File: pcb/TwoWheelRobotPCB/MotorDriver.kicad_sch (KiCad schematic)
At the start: 23 parts, among them J1 L298n_sense_connector, J2 ACS712_connector, J3 Motor1, J4 Motor2, U2 L298HN, U3 PCF8574, U4 TXB0108DQSR

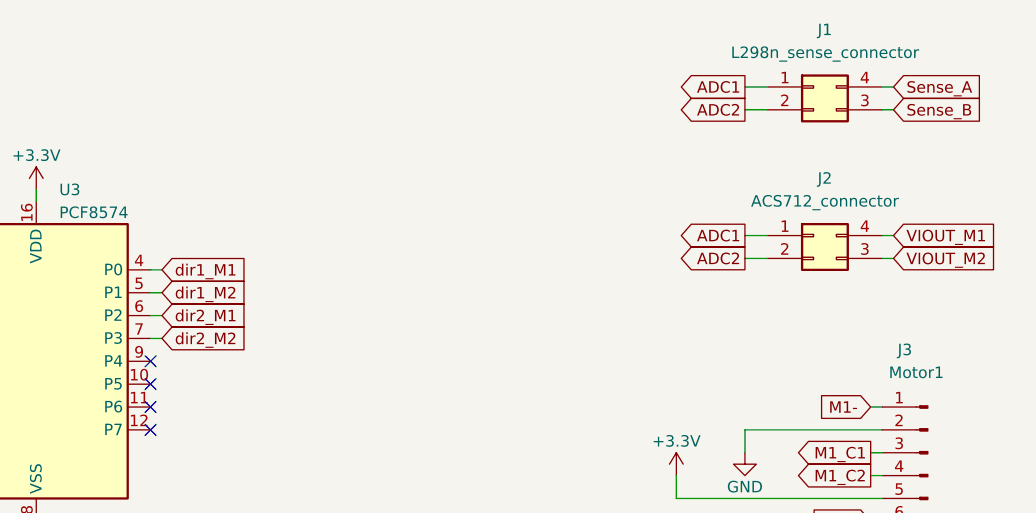
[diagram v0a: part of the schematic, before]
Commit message: update pcb
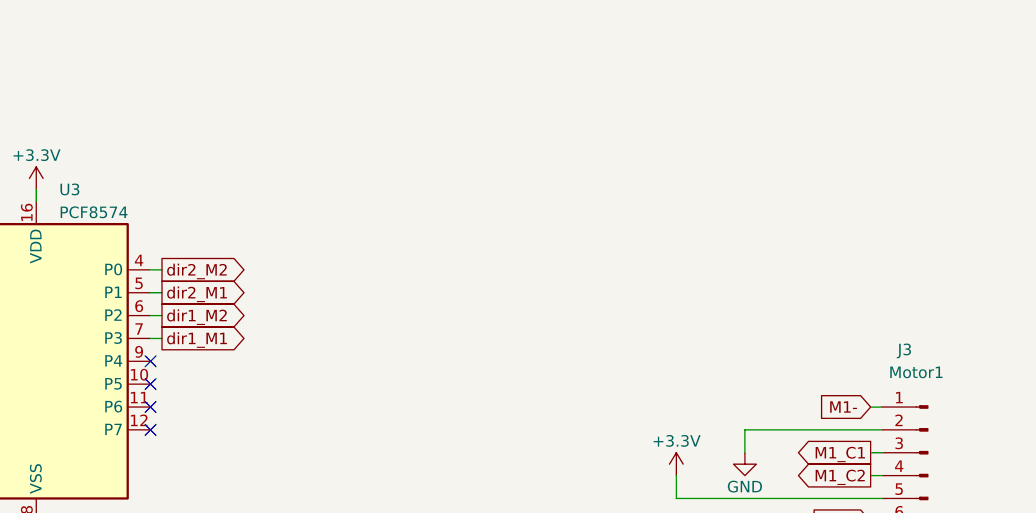
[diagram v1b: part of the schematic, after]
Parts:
- removed J1: L298n_sense_connector, Connector_PinHeader_2.54mm:PinHeader_2x02_P2.54mm_Vertical, symbol Connector_Generic:Conn_02x02_Counter_Clockwise
- removed J2: ACS712_connector, Connector_PinHeader_2.54mm:PinHeader_2x02_P2.54mm_Vertical, symbol Connector_Generic:Conn_02x02_Counter_Clockwise
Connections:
- net dir1_M1: now also U3.7 (P3); no longer U3.4 (P0)
- net dir1_M2: now also U3.6 (P2); no longer U3.5 (P1)
- net dir2_M1: now also U3.5 (P1); no longer U3.6 (P2)
- net dir2_M2: now also U3.4 (P0); no longer U3.7 (P3)
